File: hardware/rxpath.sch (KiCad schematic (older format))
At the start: 18 parts

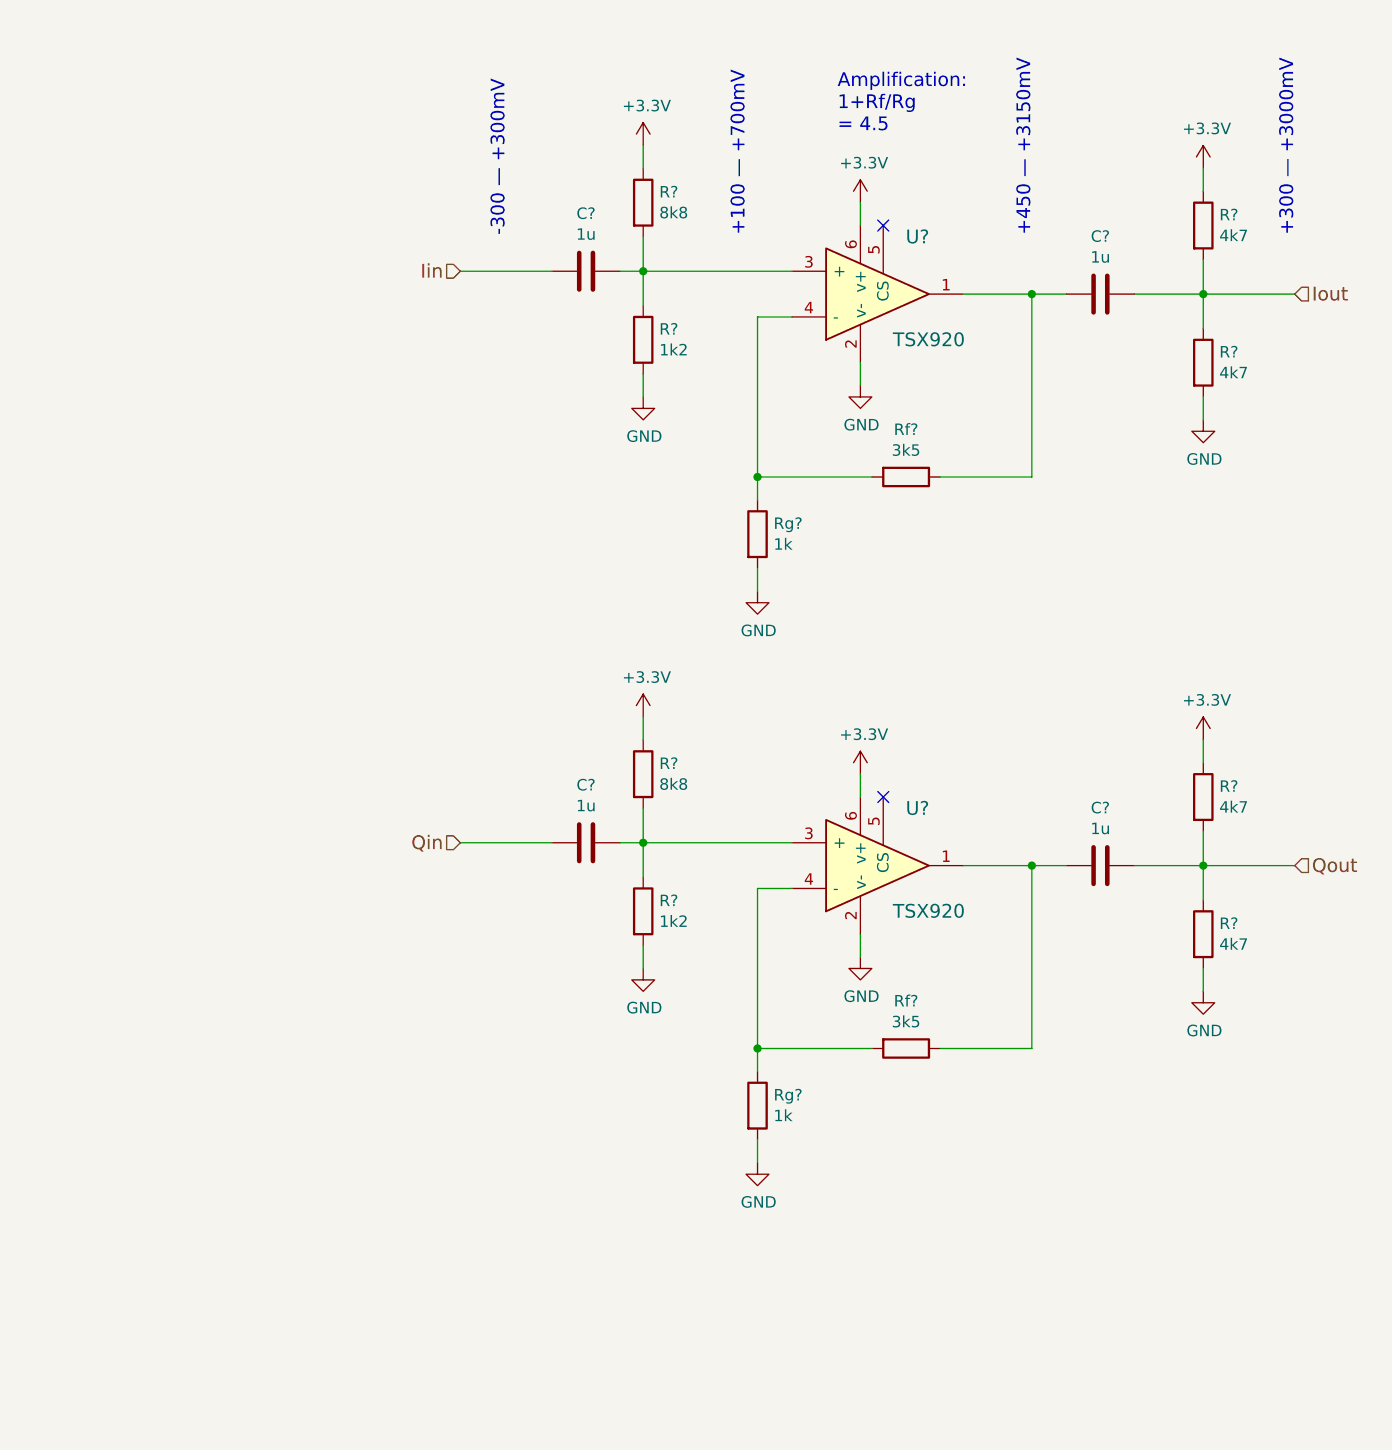
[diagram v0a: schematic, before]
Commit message: updated schematic to current
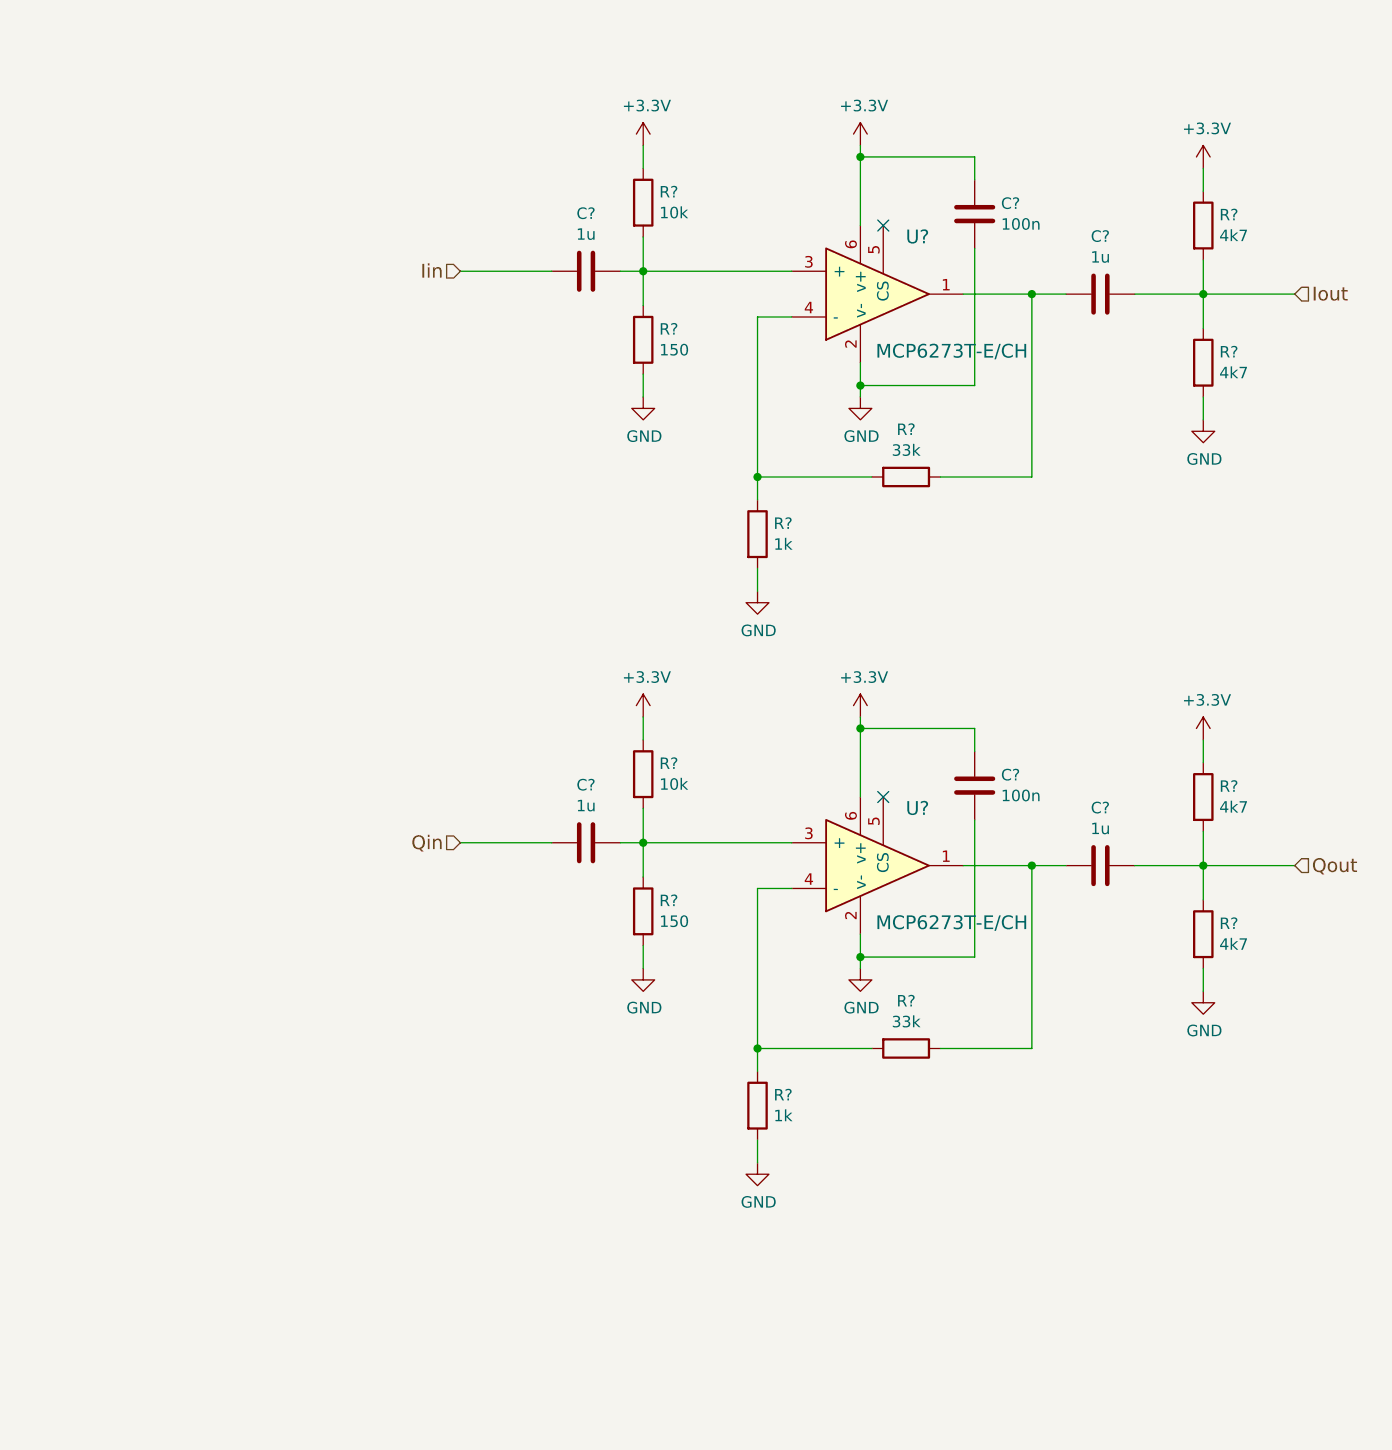
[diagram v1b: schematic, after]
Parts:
- added C? (x2): 100n, symbol C
- R? (x2): value 8k8 -> 10k
- R? (x2): value 1k2 -> 150
- R? (x2): renamed from Rf?; value 3k5 -> 33k
- U? (x2): value TSX920 -> MCP6273T-E/CH
- gave numbers to parts that had none: 1
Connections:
- net +3V3: now also C?.1, C?.1
- net GND: now also C?.2, C?.2
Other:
- note removed: "+100 — +700mV"
- note removed: "+300 — +3000mV"
- note removed: "+450 — +3150mV"
- note removed: "-300 — +300mV"
- note removed: "Amplification:\n1+Rf/Rg\n= 4.5"
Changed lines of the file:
@@
-EESchema Schematic File Version 2
+EESchema Schematic File Version 3
 LIBS:power
 LIBS:device
-LIBS:transistors
-LIBS:conn
 LIBS:linear
 LIBS:regul
-LIBS:74xx
-LIBS:cmos4000
 LIBS:adc-dac
 LIBS:memory
@@
 LIBS:digital-audio
 LIBS:philips
-LIBS:display
 LIBS:cypress
 LIBS:siliconi
@@
 LIBS:atmel
 LIBS:contrib
-LIBS:valves
 LIBS:atmel_local
 LIBS:irf
@@
 LIBS:toshiba
 LIBS:wurstradar-cache
-EELAYER 25 0
+EELAYER 26 0
 EELAYER END
 $Descr A4 11693 8268
@@
 P 4650 2250
 F 0 "R?" H 4720 2296 50  0000 L CNN
-F 1 "8k8" H 4720 2205 50  0000 L CNN
+F 1 "10k" H 4720 2205 50  0000 L CNN
 F 2 "" V 4580 2250 50  0001 C CNN
 F 3 "" H 4650 2250 50  0001 C CNN
@@
 P 4650 2850
 F 0 "R?" H 4720 2896 50  0000 L CNN
-F 1 "1k2" H 4720 2805 50  0000 L CNN
+F 1 "150" H 4720 2805 50  0000 L CNN
 F 2 "" V 4580 2850 50  0001 C CNN
 F 3 "" H 4650 2850 50  0001 C CNN
@@
 $EndComp
 Wire Wire Line
-	4650 2400 4650 2550
-Wire Wire Line
-	4650 2550 4650 2700
+	4650 2400 4650 2700
 Wire Wire Line
 	3850 2550 4250 2550
 Wire Wire Line
-	4550 2550 4650 2550
-Wire Wire Line
-	4650 2550 5300 2550
+	4550 2550 5300 2550
 Connection ~ 4650 2550
 $Comp
 L +3.3V #PWR?
 U 1 1 5A8CBF76
-P 5600 2250
-F 0 "#PWR?" H 5600 2100 50  0001 C CNN
-F 1 "+3.3V" H 5615 2423 50  0000 C CNN
-F 2 "" H 5600 2250 50  0001 C CNN
-F 3 "" H 5600 2250 50  0001 C CNN
-	1    5600 2250
+P 5600 2000
+F 0 "#PWR?" H 5600 1850 50  0001 C CNN
+F 1 "+3.3V" H 5615 2173 50  0000 C CNN
+F 2 "" H 5600 2000 50  0001 C CNN
+F 3 "" H 5600 2000 50  0001 C CNN
+	1    5600 2000
 	1    0    0    -1
 $EndComp
@@
 L GND #PWR?
 U 1 1 5A8CBF7C
-P 5600 3050
-F 0 "#PWR?" H 5600 2800 50  0001 C CNN
-F 1 "GND" H 5605 2877 50  0000 C CNN
-F 2 "" H 5600 3050 50  0001 C CNN
-F 3 "" H 5600 3050 50  0001 C CNN
-	1    5600 3050
+P 5600 3100
+F 0 "#PWR?" H 5600 2850 50  0001 C CNN
+F 1 "GND" H 5605 2927 50  0000 C CNN
+F 2 "" H 5600 3100 50  0001 C CNN
+F 3 "" H 5600 3100 50  0001 C CNN
+	1    5600 3100
 	1    0    0    -1
 $EndComp
@@
 	5300 2750 5150 2750
 Wire Wire Line
-	5150 2750 5150 3450
-Wire Wire Line
-	5150 3450 5150 3550
-$Comp
-L R Rg?
+	5150 2750 5150 3550
+$Comp
+L R R?
 U 1 1 5A8CBF85
 P 5150 3700
-F 0 "Rg?" H 5220 3746 50  0000 L CNN
+F 0 "R?" H 5220 3746 50  0000 L CNN
 F 1 "1k" H 5220 3655 50  0000 L CNN
 F 2 "" V 5080 3700 50  0001 C CNN
@@
 $EndComp
 $Comp
-L R Rf?
+L R R?
 U 1 1 5A8CBF8C
 P 5800 3450
-F 0 "Rf?" V 5593 3450 50  0000 C CNN
-F 1 "3k5" V 5684 3450 50  0000 C CNN
+F 0 "R?" V 5593 3450 50  0000 C CNN
+F 1 "33k" V 5684 3450 50  0000 C CNN
 F 2 "" V 5730 3450 50  0001 C CNN
 F 3 "" H 5800 3450 50  0001 C CNN
@@
 	6350 3450 6350 2650
 Wire Wire Line
-	6800 2650 7100 2650
-Wire Wire Line
-	7100 2650 7500 2650
+	6800 2650 7500 2650
 $Comp
 L R R?
@@
 $EndComp
 Wire Wire Line
-	7100 2500 7100 2650
-Wire Wire Line
-	7100 2650 7100 2800
+	7100 2500 7100 2800
 Connection ~ 7100 2650
 Connection ~ 6350 2650
-Text Notes 4050 2400 1    60   ~ 0
--300 — +300mV
 $Comp
 L C C?
@@
 $EndComp
 Wire Wire Line
-	6050 2650 6350 2650
-Wire Wire Line
-	6350 2650 6500 2650
-Text Notes 5100 2400 1    60   ~ 0
-+100 — +700mV
+	6050 2650 6500 2650
 $Comp
 L GND #PWR?
@@
 	1    0    0    -1
 $EndComp
-Text Notes 5500 1950 0    60   ~ 0
-Amplification:\n1+Rf/Rg\n= 4.5
-Text Notes 6350 2400 1    60   ~ 0
-+450 — +3150mV
-Text Notes 7500 2400 1    60   ~ 0
-+300 — +3000mV
 Wire Wire Line
 	4650 3000 4650 3100
@@
 	7100 3200 7100 3100
 Wire Wire Line
-	5600 3050 5600 2950
+	5600 3100 5600 2950
 Wire Wire Line
 	7100 2100 7100 2200
 Wire Wire Line
-	5600 2250 5600 2350
+	5600 2000 5600 2350
 Wire Wire Line
 	4650 2100 4650 2000
@@
 P 5650 2650
 F 0 "U?" H 5850 2900 60  0000 C CNN
-F 1 "TSX920" H 5900 2450 60  0000 C CNN
+F 1 "MCP6273T-E/CH" H 6000 2400 60  0000 C CNN
 F 2 "TO_SOT_Packages_SMD:SOT-23-6" H 5900 2350 60  0001 C CNN
 F 3 "" H 5650 2650 60  0001 C CNN
@@
 P 4650 4750
 F 0 "R?" H 4720 4796 50  0000 L CNN
-F 1 "8k8" H 4720 4705 50  0000 L CNN
+F 1 "10k" H 4720 4705 50  0000 L CNN
 F 2 "" V 4580 4750 50  0001 C CNN
 F 3 "" H 4650 4750 50  0001 C CNN
@@
 P 4650 5350
 F 0 "R?" H 4720 5396 50  0000 L CNN
-F 1 "1k2" H 4720 5305 50  0000 L CNN
+F 1 "150" H 4720 5305 50  0000 L CNN
 F 2 "" V 4580 5350 50  0001 C CNN
 F 3 "" H 4650 5350 50  0001 C CNN
@@
 $EndComp
 Wire Wire Line
-	4650 4900 4650 5050
-Wire Wire Line
-	4650 5050 4650 5200
+	4650 4900 4650 5200
 Wire Wire Line
 	3850 5050 4250 5050
 Wire Wire Line
-	4550 5050 4650 5050
-Wire Wire Line
-	4650 5050 5300 5050
+	4550 5050 5300 5050
 Connection ~ 4650 5050
 $Comp
 L +3.3V #PWR?
 U 1 1 5A8CC820
-P 5600 4750
-F 0 "#PWR?" H 5600 4600 50  0001 C CNN
-F 1 "+3.3V" H 5615 4923 50  0000 C CNN
-F 2 "" H 5600 4750 50  0001 C CNN
-F 3 "" H 5600 4750 50  0001 C CNN
-	1    5600 4750
+P 5600 4500
+F 0 "#PWR?" H 5600 4350 50  0001 C CNN
+F 1 "+3.3V" H 5615 4673 50  0000 C CNN
+F 2 "" H 5600 4500 50  0001 C CNN
+F 3 "" H 5600 4500 50  0001 C CNN
+	1    5600 4500
 	1    0    0    -1
 $EndComp
@@
 L GND #PWR?
 U 1 1 5A8CC826
-P 5600 5550
-F 0 "#PWR?" H 5600 5300 50  0001 C CNN
-F 1 "GND" H 5605 5377 50  0000 C CNN
-F 2 "" H 5600 5550 50  0001 C CNN
-F 3 "" H 5600 5550 50  0001 C CNN
-	1    5600 5550
+P 5600 5600
+F 0 "#PWR?" H 5600 5350 50  0001 C CNN
+F 1 "GND" H 5605 5427 50  0000 C CNN
+F 2 "" H 5600 5600 50  0001 C CNN
+F 3 "" H 5600 5600 50  0001 C CNN
+	1    5600 5600
 	1    0    0    -1
 $EndComp
@@
 	5300 5250 5150 5250
 Wire Wire Line
-	5150 5250 5150 5950
-Wire Wire Line
-	5150 5950 5150 6050
-$Comp
-L R Rg?
+	5150 5250 5150 6050
+$Comp
+L R R?
 U 1 1 5A8CC82F
 P 5150 6200
-F 0 "Rg?" H 5220 6246 50  0000 L CNN
+F 0 "R?" H 5220 6246 50  0000 L CNN
 F 1 "1k" H 5220 6155 50  0000 L CNN
 F 2 "" V 5080 6200 50  0001 C CNN
@@
 $EndComp
 $Comp
-L R Rf?
+L R R?
 U 1 1 5A8CC836
 P 5800 5950
-F 0 "Rf?" V 5593 5950 50  0000 C CNN
-F 1 "3k5" V 5684 5950 50  0000 C CNN
+F 0 "R?" V 5593 5950 50  0000 C CNN
+F 1 "33k" V 5684 5950 50  0000 C CNN
 F 2 "" V 5730 5950 50  0001 C CNN
 F 3 "" H 5800 5950 50  0001 C CNN
@@
 	6350 5950 6350 5150
 Wire Wire Line
-	6800 5150 7100 5150
-Wire Wire Line
-	7100 5150 7500 5150
+	6800 5150 7500 5150
 $Comp
 L R R?
@@
 $EndComp
 Wire Wire Line
-	7100 5000 7100 5150
-Wire Wire Line
-	7100 5150 7100 5300
+	7100 5000 7100 5300
 Connection ~ 7100 5150
 Connection ~ 6350 5150
@@
 $EndComp
 Wire Wire Line
-	6050 5150 6350 5150
-Wire Wire Line
-	6350 5150 6500 5150
+	6050 5150 6500 5150
 $Comp
 L GND #PWR?
@@
 	7100 5700 7100 5600
 Wire Wire Line
-	5600 5550 5600 5450
+	5600 5600 5600 5450
 Wire Wire Line
 	7100 4600 7100 4700
 Wire Wire Line
-	5600 4750 5600 4850
+	5600 4500 5600 4850
 Wire Wire Line
 	4650 4600 4650 4500
@@
 P 5650 5150
 F 0 "U?" H 5850 5400 60  0000 C CNN
-F 1 "TSX920" H 5900 4950 60  0000 C CNN
+F 1 "MCP6273T-E/CH" H 6000 4900 60  0000 C CNN
 F 2 "TO_SOT_Packages_SMD:SOT-23-6" H 5900 4850 60  0001 C CNN
 F 3 "" H 5650 5150 60  0001 C CNN
@@
 Text HLabel 7500 5150 2    60   Input ~ 0
 Qout
+$Comp
+L C C?
+U 1 1 5A95AB4C
+P 6100 2300
+F 0 "C?" H 6215 2346 50  0000 L CNN
+F 1 "100n" H 6215 2255 50  0000 L CNN
+F 2 "" H 6138 2150 50  0001 C CNN
+F 3 "" H 6100 2300 50  0001 C CNN
+	1    6100 2300
+	1    0    0    -1
+$EndComp
+$Comp
+L C C?
+U 1 1 5A95AE07
+P 6100 4800
+F 0 "C?" H 6215 4846 50  0000 L CNN
+F 1 "100n" H 6215 4755 50  0000 L CNN
+F 2 "" H 6138 4650 50  0001 C CNN
+F 3 "" H 6100 4800 50  0001 C CNN
+	1    6100 4800
+	1    0    0    -1
+$EndComp
+Wire Wire Line
+	6100 4650 6100 4550
+Wire Wire Line
+	6100 4550 5600 4550
+Connection ~ 5600 4550
+Wire Wire Line
+	6100 2150 6100 2050
+Wire Wire Line
+	6100 2050 5600 2050
+Connection ~ 5600 2050
+Wire Wire Line
+	6100 4950 6100 5550
+Wire Wire Line
+	6100 5550 5600 5550
+Connection ~ 5600 5550
+Wire Wire Line
+	6100 2450 6100 3050
+Wire Wire Line
+	6100 3050 5600 3050
+Connection ~ 5600 3050
 $EndSCHEMATC

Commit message: for long-term documentation: cleanup and port schematic to Kicad v5.1.4 and also export as PDF.
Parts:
- removed C? (x4): 1u, symbol C
- removed C? (x2): 100n, symbol C
- removed R? (x2): 10k, symbol R
- removed R? (x2): 150, symbol R
- removed R? (x2): 1k, symbol R
- removed R? (x2): 33k, symbol R
- removed R? (x4): 4k7, symbol R
- removed U?: MCP6273T-E/CH, TO_SOT_Packages_SMD:SOT-23-6, symbol TSX920
- added C? (x4): 1u, symbol Device:C
- added C? (x2): 100n, symbol Device:C
- added R? (x4): 4k7, symbol Device:R
- added R? (x2): 10k, symbol Device:R
- added R? (x2): 150, symbol Device:R
- added R? (x2): 33k, symbol Device:R
- added R? (x2): 1k, symbol Device:R
- added U?: MCP6273T-E/CH, TO_SOT_Packages_SMD:SOT-23-6, symbol st1:TSX920
- U?: symbol TSX920 -> st1:TSX920
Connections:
- net +3V3: now also C?.1, C?.1, R?.1, R?.1, R?.1, R?.1, U?.6 (v+)
- net GND: now also C?.2, C?.2, R?.2, R?.2, R?.2, R?.2, R?.2, R?.2, U?.2 (v-)
- net Iin: now also C?.1
- net Iout: now also C?.2, R?.1, R?.2
- net Qin: now also C?.1
- net Qout: now also C?.2, R?.1, R?.2
- net at U?.3 (+): now also C?.2, R?.1, R?.2
- net at U?.4 (-): now also R?.1, R?.1
- net at U?.1: now also C?.1, R?.2
- new net: C?.1, R?.2, U?.1
- new net: C?.2, R?.1, R?.2, U?.3 (+)
- new net: R?.1, R?.1, U?.4 (-)
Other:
- moved on the sheet: U?
